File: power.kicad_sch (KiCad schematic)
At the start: 28 parts, among them J3 Conn_01x02, Q2 AO3401A, SW8 SW_Slide_DPDT, U3 TP4056-42-ESOP8, U4 INA219AxDCN, U7 TPS62160DGK

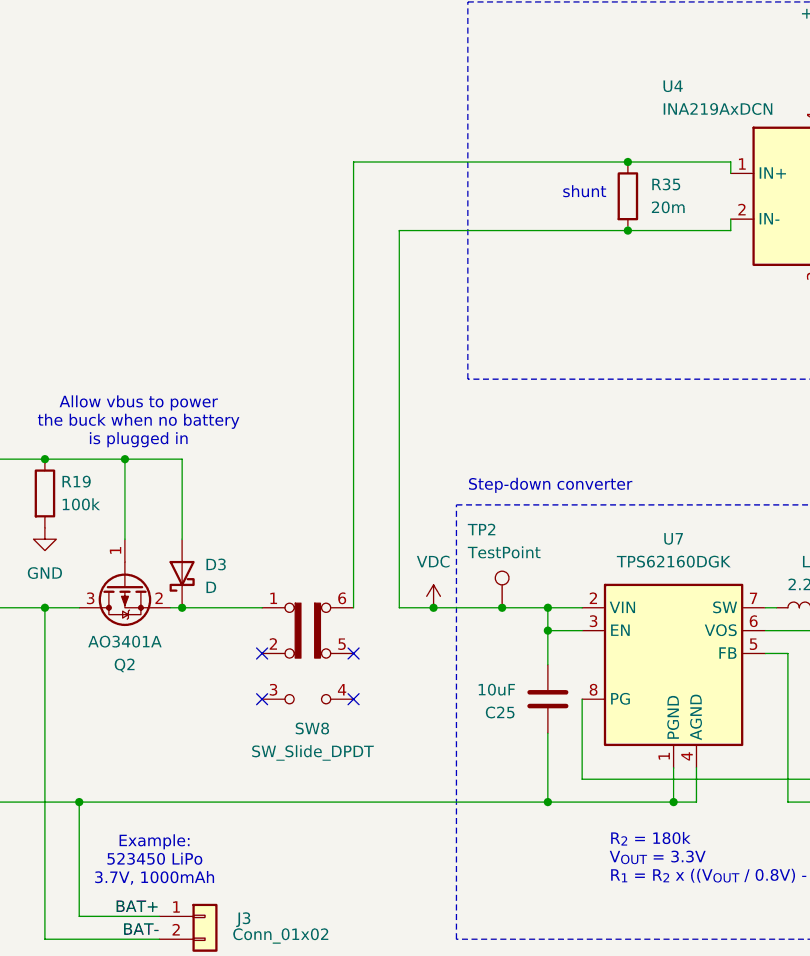
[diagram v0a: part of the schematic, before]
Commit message: fix on/off switch routing
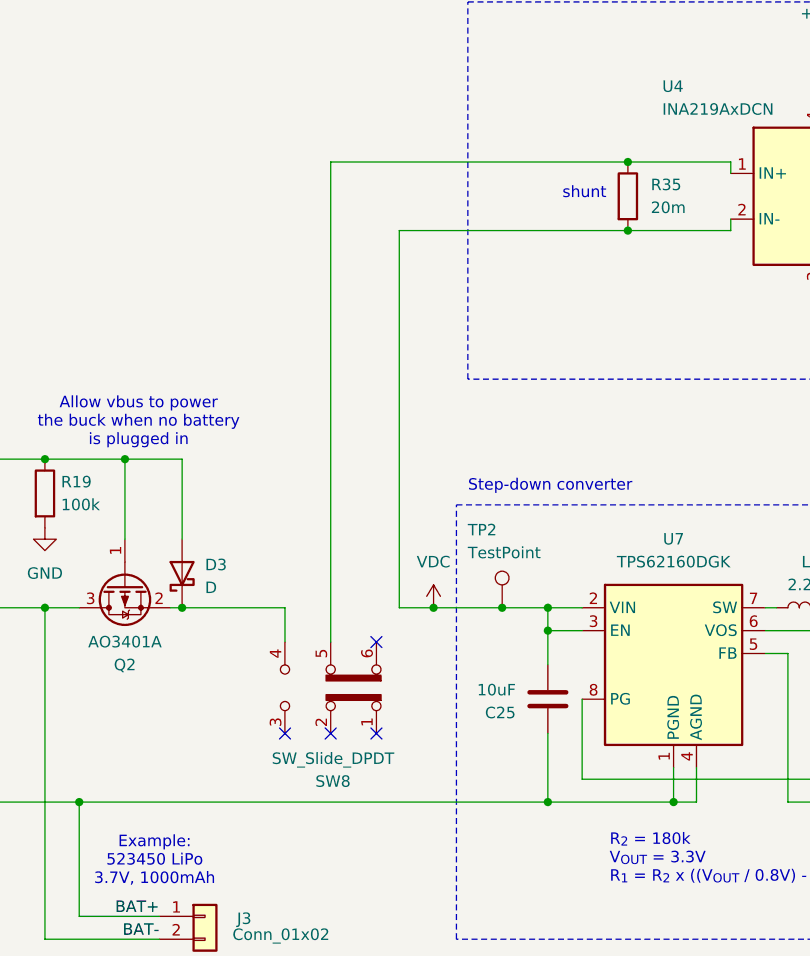
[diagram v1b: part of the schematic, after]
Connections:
- net at D3.1 (K), Q2.2 (S): now also SW8.4 (A); no longer SW8.1 (A)
- net at SW8.5 (B): now also R35.1, U4.1 (IN+)
- now unconnected: SW8.6 (C)
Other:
- moved on the sheet: SW8
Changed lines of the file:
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@@
+	)
+	(junction
+		(at 143.51 90.17)
+		(diameter 0)
+		(color 0 0 0 0)
 	)
 	(junction
@@
 	)
 	(junction
-		(at 143.51 90.17)
-		(diameter 0)
-		(color 0 0 0 0)
-	)
-	(junction
 		(at 64.77 73.66)
 		(diameter 0)
@@
 	)
 	(junction
+		(at 128.27 73.66)
+		(diameter 0)
+		(color 0 0 0 0)
+	)
+	(junction
+		(at 198.12 111.76)
+		(diameter 0)
+		(color 0 0 0 0)
+	)
+	(junction
+		(at 214.63 34.29)
+		(diameter 0)
+		(color 0 0 0 0)
+	)
+	(junction
+		(at 184.15 111.76)
+		(diameter 0)
+		(color 0 0 0 0)
+	)
+	(junction
+		(at 106.68 111.76)
+		(diameter 0)
+		(color 0 0 0 0)
+	)
+	(junction
+		(at 90.17 111.76)
+		(diameter 0)
+		(color 0 0 0 0)
+	)
+	(junction
 		(at 193.04 40.64)
 		(diameter 0)
@@
 	)
 	(junction
-		(at 128.27 73.66)
-		(diameter 0)
-		(color 0 0 0 0)
-	)
-	(junction
-		(at 198.12 111.76)
-		(diameter 0)
-		(color 0 0 0 0)
-	)
-	(junction
-		(at 214.63 34.29)
-		(diameter 0)
-		(color 0 0 0 0)
-	)
-	(junction
-		(at 184.15 111.76)
-		(diameter 0)
-		(color 0 0 0 0)
-	)
-	(junction
-		(at 106.68 111.76)
-		(diameter 0)
-		(color 0 0 0 0)
-	)
-	(junction
-		(at 90.17 111.76)
-		(diameter 0)
-		(color 0 0 0 0)
-	)
-	(junction
 		(at 137.16 73.66)
 		(diameter 0)
@@
 	)
 	(no_connect
-		(at 162.56 95.25)
+		(at 154.94 104.14)
 	)
 	(no_connect
-		(at 162.56 100.33)
+		(at 165.1 93.98)
 	)
 	(no_connect
-		(at 152.4 95.25)
+		(at 160.02 104.14)
 	)
 	(no_connect
-		(at 152.4 100.33)
+		(at 165.1 104.14)
 	)
 	(wire
@@
 	(wire
 		(pts
+			(xy 154.94 90.17) (xy 154.94 93.98)
+		)
+		(stroke
+			(width 0)
+			(type default)
+		)
+	)
+	(wire
+		(pts
 			(xy 226.06 57.15) (xy 246.38 57.15)
 		)
@@
 	(wire
 		(pts
-			(xy 162.56 40.64) (xy 162.56 90.17)
-		)
-		(stroke
-			(width 0)
-			(type default)
-		)
-	)
-	(wire
-		(pts
 			(xy 193.04 48.26) (xy 204.47 48.26)
 		)
@@
 	(wire
 		(pts
+			(xy 160.02 40.64) (xy 193.04 40.64)
+		)
+		(stroke
+			(width 0)
+			(type default)
+		)
+	)
+	(wire
+		(pts
 			(xy 184.15 111.76) (xy 198.12 111.76)
 		)
@@
 	(wire
 		(pts
+			(xy 160.02 93.98) (xy 160.02 40.64)
+		)
+		(stroke
+			(width 0)
+			(type default)
+		)
+	)
+	(wire
+		(pts
 			(xy 243.84 90.17) (xy 243.84 96.52)
 		)
@@
 	(wire
 		(pts
-			(xy 193.04 40.64) (xy 162.56 40.64)
-		)
-		(stroke
-			(width 0)
-			(type default)
-		)
-	)
-	(wire
-		(pts
-			(xy 143.51 90.17) (xy 152.4 90.17)
+			(xy 143.51 90.17) (xy 154.94 90.17)
 		)
 		(stroke
@@
 	(symbol
 		(lib_id "Switch:SW_Slide_DPDT")
-		(at 157.48 95.25 0)
+		(at 160.02 99.06 270)
+		(mirror x)
 		(unit 1)
 		(body_style 1)
@@
 		(dnp no)
 		(property "Reference" "SW8"
-			(at 157.988 103.632 0)
+			(at 160.274 109.474 90)
 			(show_name no)
 			(do_not_autoplace no)
@@
 		)
 		(property "Value" "SW_Slide_DPDT"
-			(at 157.988 106.172 0)
+			(at 160.274 106.934 90)
 			(show_name no)
 			(do_not_autoplace no)
@@
 		)
 		(property "Footprint" "Button_Switch_SMD:SW_DPDT_CK_JS202011JCQN"
-			(at 171.45 90.17 0)
+			(at 165.1 85.09 0)
 			(hide yes)
 			(show_name no)
@@
 		)
 		(property "Datasheet" ""
-			(at 157.48 95.25 0)
+			(at 160.02 99.06 0)
 			(hide yes)
 			(show_name no)
@@
 		)
 		(property "Description" "Slide Switch, dual pole double throw"
-			(at 157.48 95.25 0)
+			(at 160.02 99.06 0)
 			(hide yes)
 			(show_name no)
@@
 		)
 		(property "LCSC" "C221665"
-			(at 157.48 95.25 0)
+			(at 160.02 99.06 0)
 			(hide yes)
 			(show_name no)
@@
 		)
 		(property "Manufacturer" "C&K"
-			(at 157.48 95.25 0)
+			(at 160.02 99.06 0)
 			(hide yes)
 			(show_name no)
@@
 		)
 		(property "Manufacturer Part Number" "JS202011JCQN"
-			(at 157.48 95.25 0)
-			(hide yes)
-			(show_name no)
+			(at 160.02 99.06 0)
+			(hide yes)
+			(show_name no)
